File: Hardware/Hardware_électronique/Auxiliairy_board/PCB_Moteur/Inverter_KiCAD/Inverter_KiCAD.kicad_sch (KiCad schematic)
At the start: 71 parts, among them J1 Conn_02x02_Top_Bottom, J2 173010542, J3 Conn_02x05_Odd_Even, J4 Conn_01x02, J5 Conn_01x02, Q5 SQ2310ES, U1 MIC4606, U2 GO 10-SME/SP3, U3 GO 10-SME/SP3, U4 AZ1117-3.3, U5 MAX3097ECSE+, U7 CSD86350Q5D, U8 CSD86350Q5D

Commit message: deut routage
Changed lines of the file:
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@@
 	)
 	(rectangle
-		(start 15.24 210.82)
-		(end 193.04 13.97)
+		(start 15.24 13.97)
+		(end 193.04 210.82)
 		(stroke
 			(width 1)

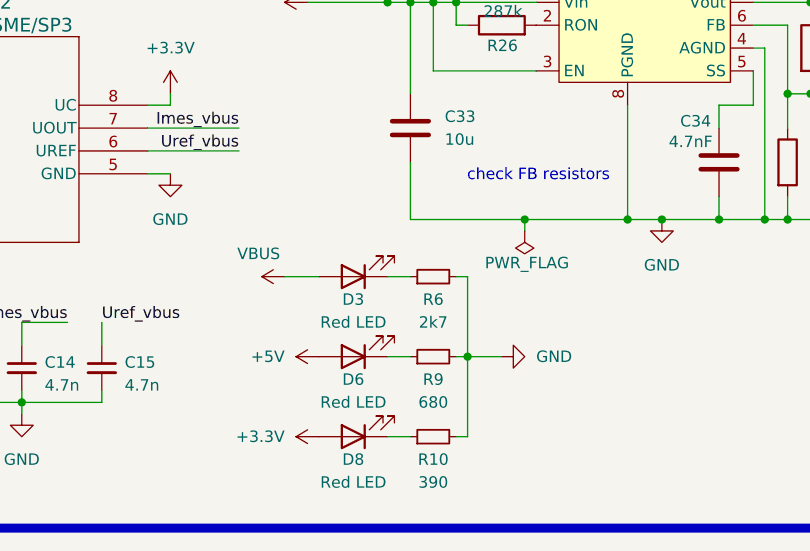
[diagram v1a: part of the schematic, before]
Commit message: almost finished pcb
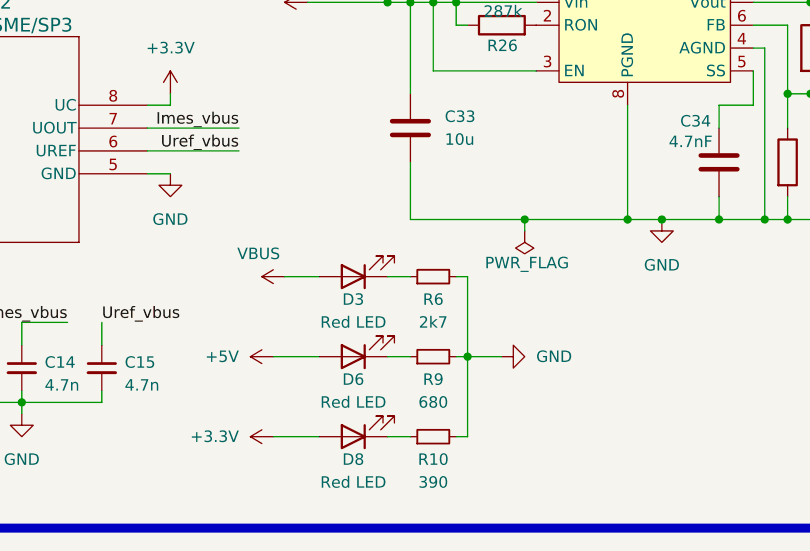
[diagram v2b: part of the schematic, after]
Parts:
- BT1: footprint (none) -> Connector_AMASS:AMASS_XT60-F_1x02_P7.20mm_Vertical
- C1, C4: footprint Capacitor_SMD:C_2220_5650Metric -> Capacitor_SMD:C_0603_1608Metric_Pad1.08x0.95mm_HandSolder
- C17: footprint Capacitor_SMD:CP_Elec_4x5.4 -> Capacitor_SMD:C_0603_1608Metric_Pad1.08x0.95mm_HandSolder
- C18: footprint Capacitor_SMD:CP_Elec_5x5.4 -> Capacitor_SMD:C_0603_1608Metric_Pad1.08x0.95mm_HandSolder
- C2, C3, C33: footprint (none) -> Capacitor_SMD:C_0603_1608Metric_Pad1.08x0.95mm_HandSolder
- C34: footprint (none) -> Capacitor_SMD:C_0402_1005Metric_Pad0.74x0.62mm_HandSolder
- C35: footprint (none) -> Capacitor_SMD:C_0402_1005Metric
- C36: footprint (none) -> Capacitor_SMD:C_0805_2012Metric
- Converter_DCDC_WPMDH1302401: footprint Custom:Converter_DCDC -> Package_TO_SOT_SMD:TO-263-7_TabPin8
- J2: footprint Buck_5V_173010542:173010542 -> Connector_PinHeader_2.54mm:PinHeader_1x03_P2.54mm_Vertical
- J3: footprint (none) -> Connector_PinHeader_2.54mm:PinHeader_2x05_P2.54mm_Vertical
- R26, R27, R28: footprint (none) -> Resistor_SMD:R_0402_1005Metric
- TP1, TP2, TP3, TP4: footprint (none) -> TestPoint:TestPoint_Pad_D2.0mm
- U1: footprint (none) -> Package_SO:TSSOP-16-1EP_4.4x5mm_P0.65mm_EP3x3mm
- U3: footprint SOIC8-GO-SME/SP3_LEM -> Custom:SOIC8-GO-SME&slash_SP3_LEM
- U7, U8: footprint DQY0008A -> CSD87351Q5D:DQY0008A
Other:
- note removed: "check FB resistors"
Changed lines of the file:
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@@
 	(wire
 		(pts
+			(xy 85.09 262.89) (xy 90.17 262.89)
+		)
+		(stroke
+			(width 0)
+			(type default)
+		)
+	)
+	(wire
+		(pts
 			(xy 242.57 187.96) (xy 243.84 187.96)
 		)
@@
 	(wire
 		(pts
+			(xy 85.09 271.78) (xy 90.17 271.78)
+		)
+		(stroke
+			(width 0)
+			(type default)
+		)
+	)
+	(wire
+		(pts
 			(xy 36.83 234.95) (xy 38.1 234.95)
 		)
@@
 		)
 	)
-	(text "check FB resistors"
-		(exclude_from_sim no)
-		(at 114.554 242.824 0)
-		(effects
-			(font
-				(size 1.27 1.27)
-			)
-		)
-	)
 	(text "STM32G474RET6 uC for signals analyse and protection\nButtons, leds, screen and rotary encoder connectors"
 		(exclude_from_sim no)
@@
 			)
 		)
-		(property "Footprint" "Buck_5V_173010542:173010542"
+		(property "Footprint" "Connector_PinHeader_2.54mm:PinHeader_1x03_P2.54mm_Vertical"
 			(at 190.5 222.25 0)
 			(effects
@@
 			)
 		)
-		(property "Footprint" ""
+		(property "Footprint" "Capacitor_SMD:C_0402_1005Metric_Pad0.74x0.62mm_HandSolder"
 			(at 135.5852 245.11 0)
 			(effects
@@
 			)
 		)
-		(property "Footprint" "DQY0008A"
+		(property "Footprint" "CSD87351Q5D:DQY0008A"
 			(at 38.1 129.54 0)
 			(effects
@@
 			)
 		)
-		(property "Footprint" ""
+		(property "Footprint" "Capacitor_SMD:C_0805_2012Metric"
 			(at 160.9852 237.49 0)
 			(effects
@@
 			)
 		)
-		(property "Footprint" ""
+		(property "Footprint" "Capacitor_SMD:C_0603_1608Metric_Pad1.08x0.95mm_HandSolder"
 			(at 77.47 66.04 0)
 			(effects
@@
 			)
 		)
-		(property "Footprint" ""
+		(property "Footprint" "Capacitor_SMD:C_0603_1608Metric_Pad1.08x0.95mm_HandSolder"
 			(at 45.72 87.63 0)
 			(effects
@@
 			)
 		)
-		(property "Footprint" "Capacitor_SMD:C_2220_5650Metric"
+		(property "Footprint" "Capacitor_SMD:C_0603_1608Metric_Pad1.08x0.95mm_HandSolder"
 			(at 125.73 115.57 0)
 			(effects
@@
 			)
 		)
-		(property "Footprint" "Capacitor_SMD:C_2220_5650Metric"
+		(property "Footprint" "Capacitor_SMD:C_0603_1608Metric_Pad1.08x0.95mm_HandSolder"
 			(at 53.34 114.3 0)
 			(effects
@@
 			)
 		)
-		(property "Footprint" ""
+		(property "Footprint" "TestPoint:TestPoint_Pad_D2.0mm"
 			(at 102.87 223.52 0)
 			(effects
@@
 			)
 		)
-		(property "Footprint" ""
+		(property "Footprint" "TestPoint:TestPoint_Pad_D2.0mm"
 			(at 176.53 257.81 0)
 			(effects
@@
 			)
 		)
-		(property "Footprint" "Capacitor_SMD:CP_Elec_4x5.4"
+		(property "Footprint" "Capacitor_SMD:C_0603_1608Metric_Pad1.08x0.95mm_HandSolder"
 			(at 169.8752 267.97 0)
 			(effects
@@
 			)
 		)
-		(property "Footprint" "DQY0008A"
+		(property "Footprint" "CSD87351Q5D:DQY0008A"
 			(at 101.6 130.81 0)
 			(effects
@@
 			)
 		)
-		(property "Footprint" "Capacitor_SMD:CP_Elec_5x5.4"
+		(property "Footprint" "Capacitor_SMD:C_0603_1608Metric_Pad1.08x0.95mm_HandSolder"
 			(at 195.2752 267.97 0)
 			(effects
@@
 			)
 		)
-		(property "Footprint" ""
+		(property "Footprint" "TestPoint:TestPoint_Pad_D2.0mm"
 			(at 198.12 257.81 0)
 			(effects
@@
 			)
 		)
-		(property "Footprint" ""
+		(property "Footprint" "Capacitor_SMD:C_0402_1005Metric"
 			(at 153.3652 232.41 0)
 			(effects
@@
 	(symbol
 		(lib_id "power:+3.3V")
-		(at 90.17 271.78 90)
+		(at 85.09 271.78 90)
 		(unit 1)
 		(exclude_from_sim no)
@@
 		(fields_autoplaced yes)
 		(property "Reference" "#PWR030"
-			(at 93.98 271.78 0)
+			(at 88.9 271.78 0)
 			(effects
 				(font
@@
 		)
 		(property "Value" "+3.3V"
-			(at 86.36 271.7799 90)
+			(at 81.28 271.7799 90)
 			(effects
 				(font
@@
 		)
 		(property "Footprint" ""
-			(at 90.17 271.78 0)
+			(at 85.09 271.78 0)
 			(effects
 				(font
@@
 		)
 		(property "Datasheet" ""
-			(at 90.17 271.78 0)
+			(at 85.09 271.78 0)
 			(effects
 				(font
@@
 		)
 		(property "Description" "Power symbol creates a global label with name \"+3.3V\""
-			(at 90.17 271.78 0)
+			(at 85.09 271.78 0)
 			(effects
 				(font
@@
 			)
 		)
-		(property "Footprint" ""
+		(property "Footprint" "TestPoint:TestPoint_Pad_D2.0mm"
 			(at 186.69 233.68 0)
 			(effects
@@
 			)
 		)
-		(property "Footprint" ""
+		(property "Footprint" "Resistor_SMD:R_0402_1005Metric"
 			(at 143.002 228.6 90)
 			(effects
@@
 			)
 		)
-		(property "Footprint" ""
+		(property "Footprint" "Connector_PinHeader_2.54mm:PinHeader_2x05_P2.54mm_Vertical"
 			(at 162.56 121.92 0)
 			(effects
@@
 			)
 		)
-		(property "Footprint" "SOIC8-GO-SME/SP3_LEM"
+		(property "Footprint" "Custom:SOIC8-GO-SME&slash_SP3_LEM"
 			(at 138.43 41.91 0)
 			(effects
@@
 			)
 		)
-		(property "Footprint" "Custom:Converter_DCDC"
+		(property "Footprint" "Package_TO_SOT_SMD:TO-263-7_TabPin8"
 			(at 128.27 228.6 0)
 			(effects
@@
 	(symbol
 		(lib_id "power:+5V")
-		(at 90.17 262.89 90)
+		(at 85.09 262.89 90)
 		(unit 1)
 		(exclude_from_sim no)
@@
 		(fields_autoplaced yes)
 		(property "Reference" "#PWR031"
-			(at 93.98 262.89 0)
+			(at 88.9 262.89 0)
 			(effects
 				(font
@@
 		)
 		(property "Value" "+5V"
-			(at 86.36 262.8899 90)
+			(at 81.28 262.8899 90)
 			(effects
 				(font
@@
 		)
 		(property "Footprint" ""
-			(at 90.17 262.89 0)
+			(at 85.09 262.89 0)
 			(effects
 				(font
@@
 		)
 		(property "Datasheet" ""
-			(at 90.17 262.89 0)
+			(at 85.09 262.89 0)
 			(effects
 				(font
@@
 		)
 		(property "Description" "Power symbol creates a global label with name \"+5V\""
-			(at 90.17 262.89 0)
+			(at 85.09 262.89 0)
 			(effects
 				(font
@@
 			)
 		)
-		(property "Footprint" ""
+		(property "Footprint" "Resistor_SMD:R_0402_1005Metric"
 			(at 140.462 241.3 90)
 			(effects
@@
 			)
 		)
-		(property "Footprint" ""
+		(property "Footprint" "Connector_AMASS:AMASS_XT60-F_1x02_P7.20mm_Vertical"
 			(at 22.86 242.316 90)
 			(effects
@@
 			)
 		)
-		(property "Footprint" ""
+		(property "Footprint" "Resistor_SMD:R_0402_1005Metric"
 			(at 110.49 227.838 90)
 			(effects
@@
 			)
 		)
-		(property "Footprint" ""
+		(property "Footprint" "Package_SO:TSSOP-16-1EP_4.4x5mm_P0.65mm_EP3x3mm"
 			(at 48.26 72.39 0)
 			(effects
@@
 			)
 		)
-		(property "Footprint" ""
+		(property "Footprint" "Capacitor_SMD:C_0603_1608Metric_Pad1.08x0.95mm_HandSolder"
 			(at 101.2952 241.3 0)
 			(effects
